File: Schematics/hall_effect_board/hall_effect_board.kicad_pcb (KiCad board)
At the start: 2 copper layers, 17.5 x 30.5 mm, 5 parts, among them J3 HALL-1, U1 TMAG5273A1QDBVT

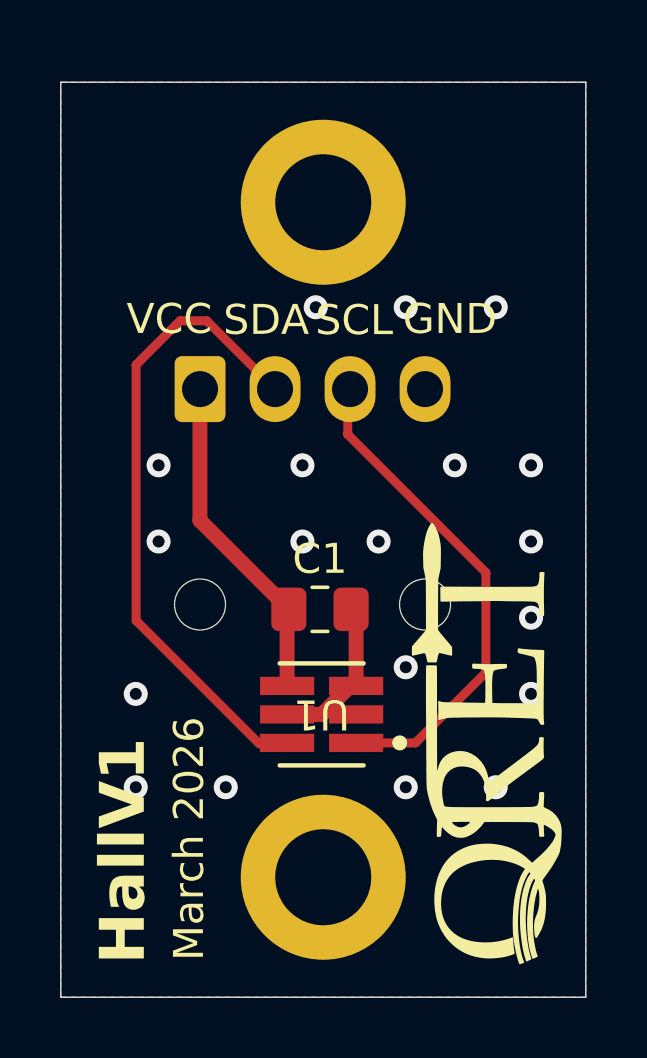
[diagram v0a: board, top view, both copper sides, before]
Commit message: Add LED
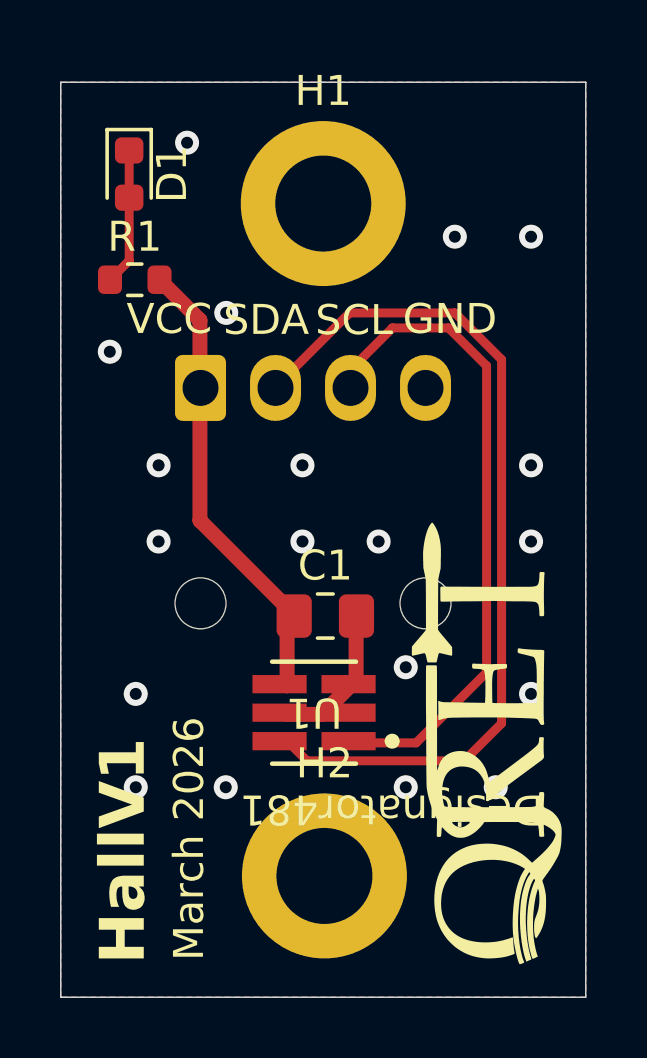
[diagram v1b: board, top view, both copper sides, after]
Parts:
- removed J3: HALL-1, Connector_Molex:Molex_Nano-Fit_105313-xx04_1x04_P2.50mm_Horizontal
- added D1: PWR_3V3_LED (GRN), LED_SMD:LED_0603_1608Metric, F.Cu at (113.6, 61.4)
- added J1: HALL-1, Connector_Molex:Molex_Nano-Fit_105313-xx04_1x04_P2.50mm_Horizontal, B.Cu at (116.0, 68.5)
- added R1: 3.3k, Resistor_SMD:R_0603_1608Metric, F.Cu at (113.8, 64.9)
- moved H2 22.5 mm to (120.1, 84.8)
- moved H1 22.5 mm to (120.1, 62.4)
- moved C1 0.29 mm to (120.1, 76.1)
- moved U1 0.26 mm to (119.8, 79.4)
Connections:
- U1 pad 6: SCA -> SDA
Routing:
- net SDA: track 0.00 -> 29.2 mm
- net SCA: track 21.5 -> 0.00 mm
- net Net-(D1-A): track 0.00 -> 4.57 mm
- net SCL: track 17.2 -> 21.3 mm
- net +3V3: track 11.7 -> 15.3 mm
